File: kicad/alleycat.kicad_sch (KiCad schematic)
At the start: 117 parts, among them J1 Conn_01x04_Male, J2 USB_C_Receptacle_USB2.0, J3 Conn_01x04_Female, SW1 SW_Push, SW2 RotaryEncoder_Switch, U1 nRF52840_holyiot_18010, U2 TP4056, U3 DW01A, U4 FS8205, U5 SRV05-4, U6 XC6206PxxxMR

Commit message: uhh uhhh uhhh uhh uhhh uhhh uhhh uuhhh uhhh uhh uhh uhhhu hh uhh footprints
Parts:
- C1, C2, C3, C4, C5, C6, C7, C8: footprint (none) -> Capacitor_SMD:C_0805_2012Metric
- D38, D39: footprint (none) -> LED_SMD:LED_0805_2012Metric
- D43: footprint (none) -> MX:SOD-323
- F1: footprint (none) -> Fuse:Fuse_1206_3216Metric
- JP1: footprint (none) -> Jumper:SolderJumper-2_P1.3mm_Open_TrianglePad1.0x1.5mm
- L1: footprint (none) -> Capacitor_SMD:C_0402_1005Metric
- R1, R10, R11, R2, R3, R4, R5, R8, R9: footprint (none) -> Resistor_SMD:R_0805_2012Metric

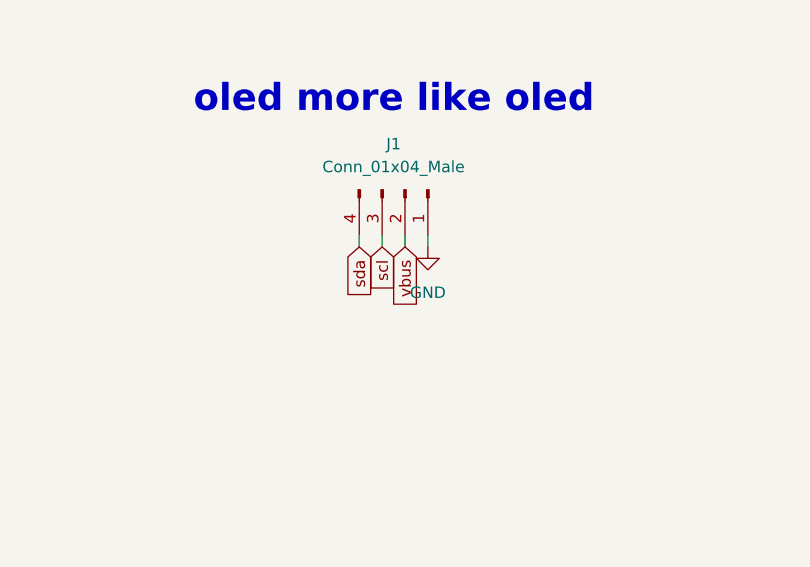
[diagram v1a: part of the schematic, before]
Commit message: pcb edit pog pog pog
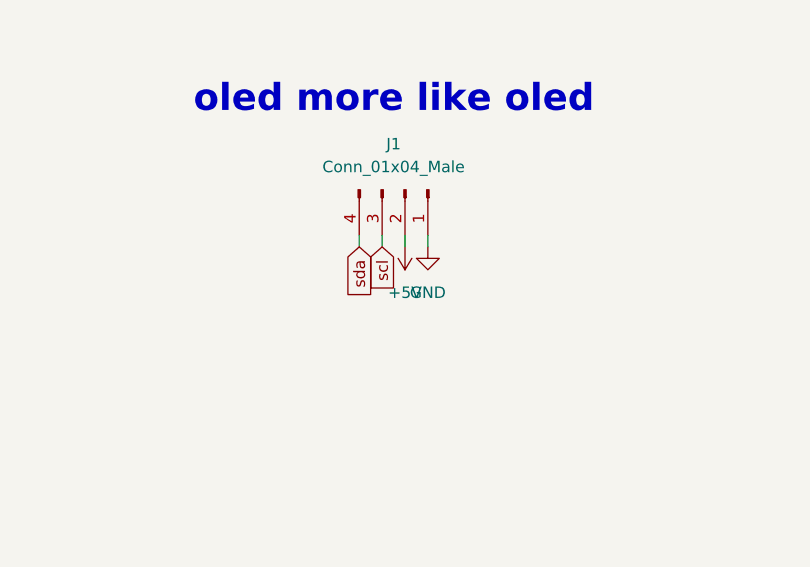
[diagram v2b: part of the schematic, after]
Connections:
- net +5V: now also J1.2 (Pin_2)
- net vbus: no longer J1.2 (Pin_2)
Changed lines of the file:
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@@
-    )
-  )
-  (global_label "vbus" (shape input) (at 45.72 266.7 270) (fields_autoplaced)
-    (effects (font (size 1.27 1.27)) (justify right))
-    (property "Intersheet References" "${INTERSHEET_REFS}" (id 0) (at 45.6406 273.4069 90)
-      (effects (font (size 1.27 1.27)) (justify right) hide)
     )
   )
@@
     (pin "1")
     (pin "2")
+  )
+  (symbol (lib_id "power:+5V") (at 45.72 266.7 180) (unit 1)
+    (in_bom yes) (on_board yes) (fields_autoplaced)
+    (property "Reference" "#PWR?" (id 0) (at 45.72 262.89 0)
+      (effects (font (size 1.27 1.27)) hide)
+    )
+    (property "Value" "+5V" (id 1) (at 45.72 271.78 0))
+    (property "Footprint" "" (id 2) (at 45.72 266.7 0)
+      (effects (font (size 1.27 1.27)) hide)
+    )
+    (property "Datasheet" "" (id 3) (at 45.72 266.7 0)
+      (effects (font (size 1.27 1.27)) hide)
+    )
+    (pin "1")
   )
   (symbol (lib_id "Device:R_Small") (at 163.83 140.97 0) (unit 1)
@@
       (reference "#PWR027") (unit 1) (value "+3.3V") (footprint "")
     )
+    (path "/cbf94107-943d-4133-8ad6-7916fb9ebd37"
+      (reference "#PWR?") (unit 1) (value "+5V") (footprint "")
+    )
     (path "/e80f4818-6806-41f2-b9c3-d610345fa90c"
